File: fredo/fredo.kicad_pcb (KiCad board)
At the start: 2 copper layers, 64 x 66 mm, 24 parts, among them J1 Conn_02x20_Odd_Even, J2 Conn_02x20_Odd_Even, Q1 DMG2305UX, Q2 DMG2305UX, U1 DRV8835DSSR

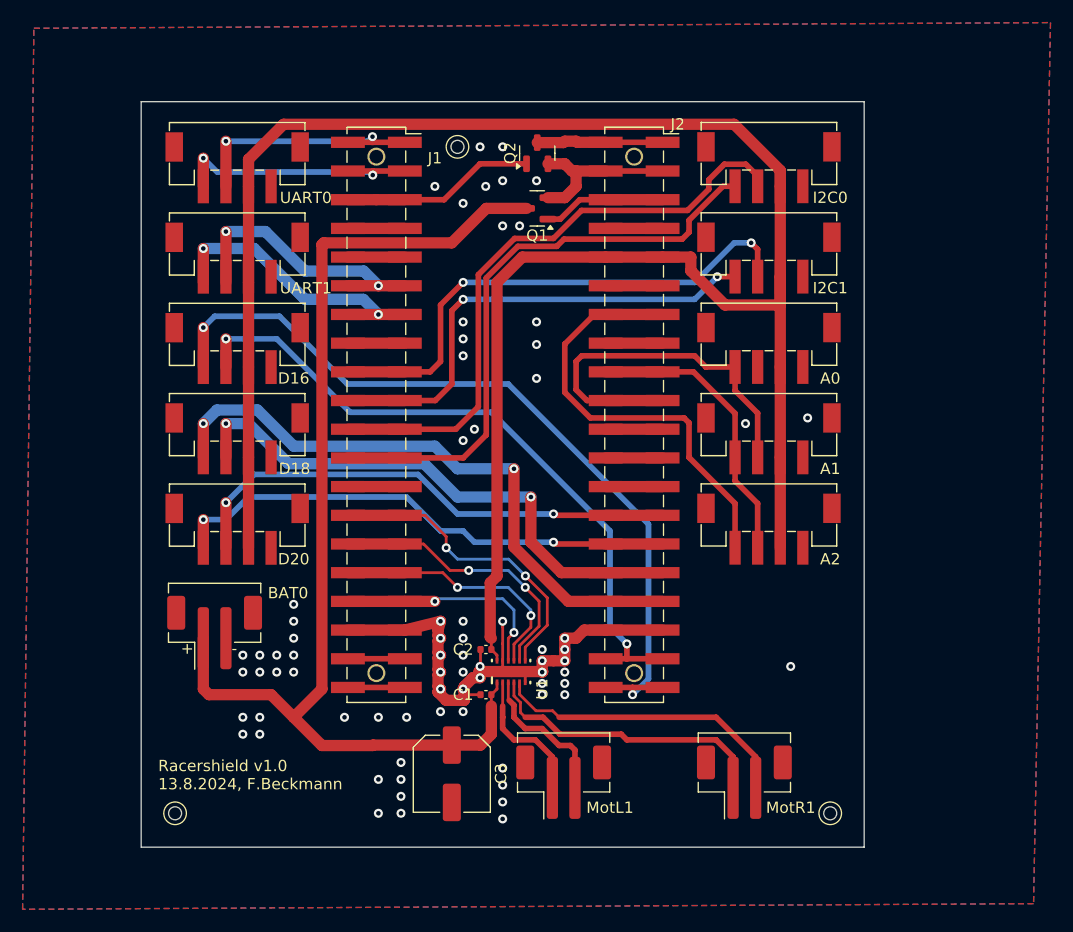
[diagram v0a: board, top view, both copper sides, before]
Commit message: Platine v1-1 mit Produktion bei JLCPCB
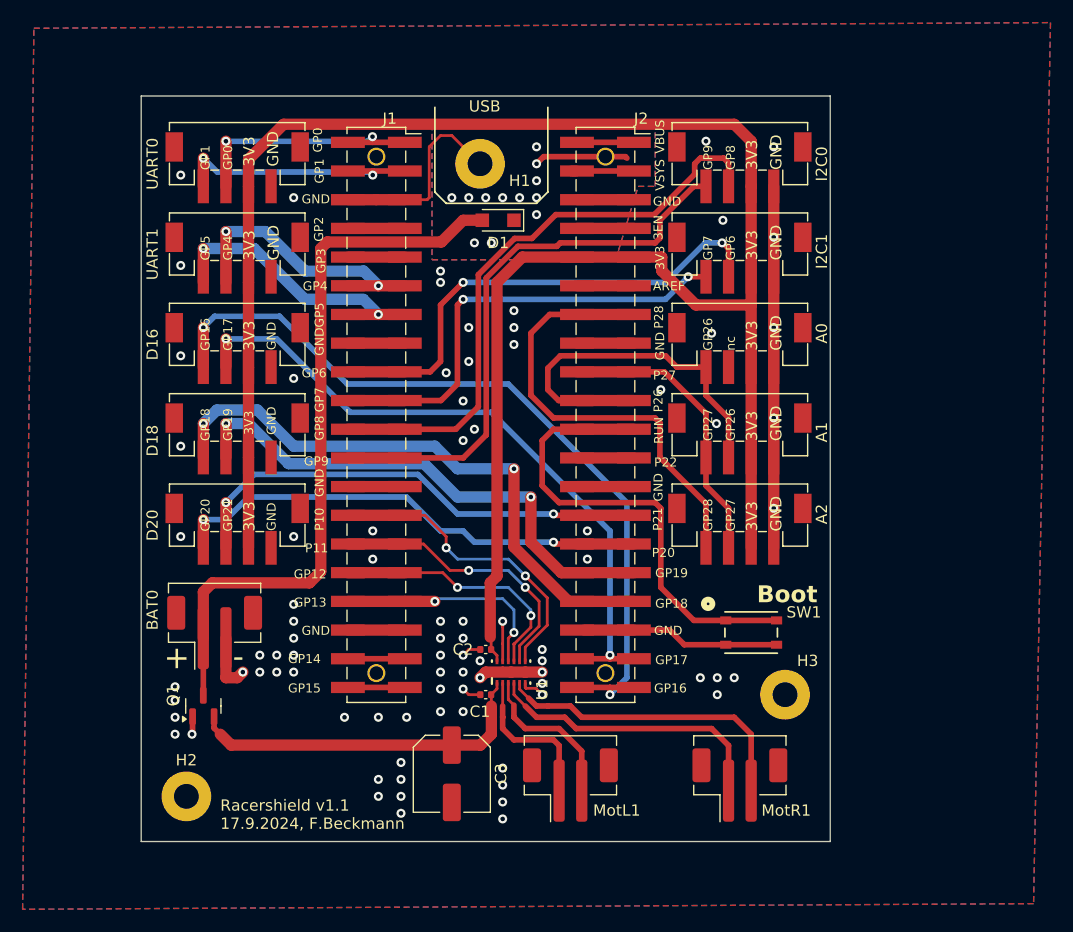
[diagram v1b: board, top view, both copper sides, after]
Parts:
- removed Q2: DMG2305UX, Package_TO_SOT_SMD:SOT-23
- removed h1, h2, h3: jlcpcb_tooling_hole, fredo:jlcpcb_tooling_hole
- added D1: PMEG2010ER, Diode_SMD:Nexperia_CFP3_SOD-123W, F.Cu at (61.6, 45.0)
- added H1: MountingHole_Pad, MountingHole:MountingHole_2.2mm_M2_Pad, F.Cu at (60.0, 40.0)
- added H2: MountingHole_Pad, MountingHole:MountingHole_2.2mm_M2_Pad, F.Cu at (34.0, 96.0)
- added H3: MountingHole_Pad, MountingHole:MountingHole_2.2mm_M2_Pad, F.Cu at (87.0, 87.0)
- added SW1: PTS815 SJM 250 SMTR LFS, fredo:SW4_PTS815 SJM 250 SMTR LFS_CNK, F.Cu at (84.0, 81.5)
- moved Q1 53.1 mm to (35.5, 88.0), turned to 90 degrees
- moved A0 2.58 mm to (83.0, 54.5)
- moved A1 2.58 mm to (83.0, 62.5)
- moved A2 2.58 mm to (83.0, 70.5)
- moved I2C0 2.58 mm to (83.0, 38.5)
- moved I2C1 2.58 mm to (83.0, 46.5)
- moved J2 2.54 mm to (71.1, 62.2)
- moved MotL1 0.65 mm to (68.0, 95.0)
- moved MotR1 0.47 mm to (83.0, 95.0)
- moved U1 0.05 mm to (62.8, 85.0)
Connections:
- C1 pad 2: VBAT -> VBATP
- C3 pad 1: VBAT -> VBATP
- J1 pad : GND -> (no net)
- J2 pad : GND -> VSYS
- Q1 pad 2: VSYS -> VBATP
- U1 pad 1: VBAT -> VBATP
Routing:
- net RUN: track 5.04 -> 42.3 mm
- net VBAT: track 99.6 -> 64.2 mm
- net VBATP: track 0.00 -> 31.4 mm
- net GND: track 101.5 -> 122.0 mm, vias 74 -> 85
- net VBUS: track 11.2 -> 5.04 mm
- net 3V3: track 182.8 -> 176.8 mm
- net GP21: track 45.2 -> 42.7 mm
- net GP20: track 45.7 -> 43.2 mm
- net GP19: track 49.5 -> 46.9 mm
- net GP18: track 55.2 -> 52.7 mm
- net I2C1_SDA/GP6: track 46.6 -> 44.1 mm
- net I2C0_SCL/GP9: track 53.0 -> 50.7 mm
- net I2C1_SCL/GP7: track 42.6 -> 40.4 mm
- net GP16: track 73.3 -> 71.6 mm
- net ADC2/GP28: track 38.9 -> 40.5 mm
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- added copper zone on B.Cu, net VSYS
- added copper zone on F.Cu, net VSYS
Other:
- board size 64 x 66 mm -> 61 x 66 mm
- board text added: "3EN"
- board text added: "3V3"
- board text added: "AREF"
- board text added: "Boot"
- board text added: "GND"
- board text added: "GP0"
- board text added: "GP1"
- board text added: "GP12"
- board text added: "GP13"
- board text added: "GP14"
- board text added: "GP15"
- board text added: "GP16"
- board text added: "GP17"
- board text added: "GP18"
- board text added: "GP19"
- board text added: "GP2"
- board text added: "GP20"
- board text added: "GP21"
- board text added: "GP26"
- board text added: "GP27"
- board text added: "GP28"
- board text added: "GP3"
- board text added: "GP4"
- board text added: "GP5"
- board text added: "GP6"
- board text added: "GP7"
- board text added: "GP8"
- board text added: "GP9"
- board text added: "P10"
- board text added: "P11"
- board text added: "P20"
- board text added: "P21"
- board text added: "P22"
- board text added: "P26"
- board text added: "P27"
- board text added: "P28"
- board text added: "RUN"
- board text added: "Racershield v1.1 17.9.2024, F.Beckmann"
- board text added: "USB"
- board text added: "VBUS"
- board text added: "VSYS"
- board text added: "nc"
- board text removed: "Racershield v1.0 13.8.2024, F.Beckmann"
